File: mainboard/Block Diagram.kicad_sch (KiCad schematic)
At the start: 0 parts

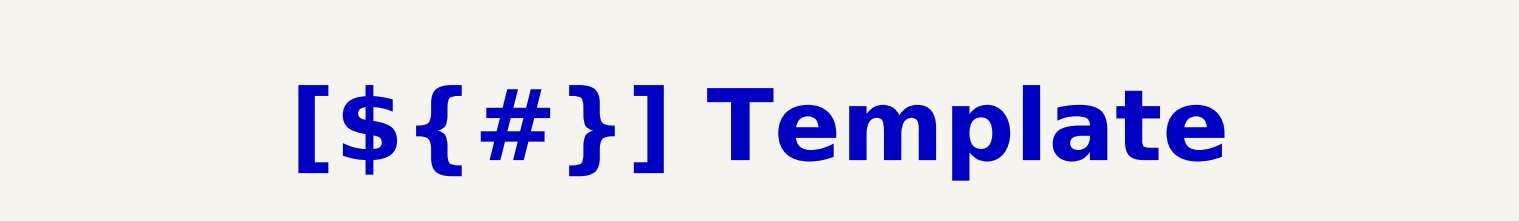
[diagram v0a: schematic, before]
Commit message: Layout complete
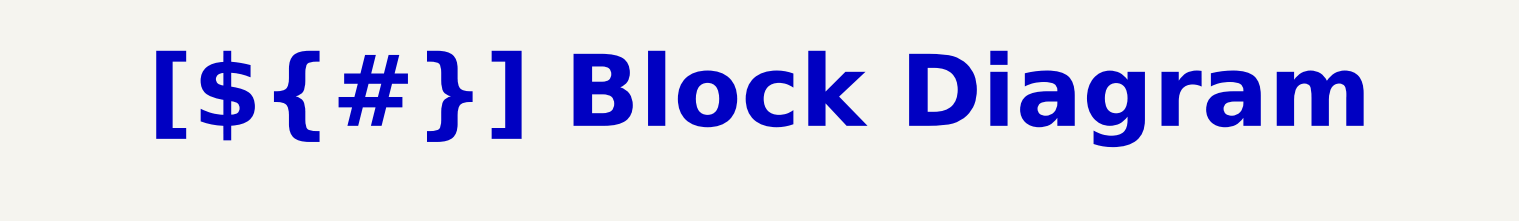
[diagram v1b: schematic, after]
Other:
- title: Template -> Block Diagram
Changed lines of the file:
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@@
 	(paper "A3")
 	(title_block
-		(title "Template")
+		(title "Block Diagram")
 		(date "2025-12-19")
 		(rev "1")
@@
 	(text_box "[${#}] ${TITLE}"
 		(exclude_from_sim no)
-		(at 144.78 20.32 0)
-		(size 130.81 12.7)
+		(at 12.7 12.7 0)
+		(size 394.97 20.32)
 		(margins 5.9999 5.9999 5.9999 5.9999)
 		(stroke
